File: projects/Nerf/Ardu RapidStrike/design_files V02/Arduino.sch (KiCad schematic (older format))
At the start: 51 parts, among them J1 BATT_IN, J10 MTR_2, J11 BATT_OUT, J12 CLIP, J13 NPTH, J14 NPTH, J16 NPTH, J2 BATT_IN, J3 PUSHER, J4 JAM, J5 I2C, J6 TRIGGER, J7 FTDI, J8 SENSORS, J9 MTR_1, Q1 IRLB8721, SW1 SW_Rotary8, SW2 SW_Push, U1 MCP1702, U2 L293D, U3 HALL SENSOR, U4 HALL SENSOR, U5 ATMEGA328P-PU, U6 HALL SENSOR, Y1 16Mhz

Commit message: Updates
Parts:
- removed J6: TRIGGER, Connectors_Molex:Molex_PicoBlade_53048-0610_06x1.25mm_Angled, symbol Conn_01x06
- removed SW2: SW_Push, footprints:SW_PUSH_6mm, symbol SW_Push
- added C9, C?: 0.1uF, footprints:C_Disc_D3.4mm_W2.1mm_P2.50mm, symbol C
- added J15: BATT, Connectors_Terminal_Blocks:TerminalBlock_bornier-2_P5.08mm, symbol Conn_01x02
- added J17: PSH_IN, footprints:Molex_PicoBlade_53048-0410_04x1.25mm_Angled, symbol Conn_01x04
- added J18: PSH_OUT, footprints:Molex_PicoBlade_53048-0410_04x1.25mm_Angled, symbol Conn_01x04
- added J?: TRIG, Pin_Headers:Pin_Header_Straight_2x01_Pitch2.00mm, symbol Conn_01x02
- added J?: REV, Pin_Headers:Pin_Header_Straight_2x01_Pitch2.00mm, symbol Conn_01x02
- added J?: PUSH, Pin_Headers:Pin_Header_Straight_2x01_Pitch2.00mm, symbol Conn_01x02
- added J?: BUTTON, Pin_Headers:Pin_Header_Straight_2x01_Pitch2.00mm, symbol Conn_01x02
- added J? (x2): TRIG_OUT, Connectors_Molex:Molex_PicoBlade_53048-0610_06x1.25mm_Angled, symbol Conn_01x06
- added R17, R?: 10K, footprints:R__P5.08mm, symbol R
- added R?: 1K, footprints:R__P5.08mm, symbol R
- added U7, U?: 74LS14, Housings_DIP:DIP-8_W7.62mm, symbol 74LS14
- J3: footprint footprints:TerminalBlock_Phoenix_PT-1,5-2-3.5-H_1x02_P3.50mm_Horizontal -> Connectors_Terminal_Blocks:TerminalBlock_bornier-2_P5.08mm
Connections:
- net labels added: #RTS, BUTTON, PUSHER, REV
- net labels removed: ACCEL, PUSH
- wire segments 209 -> 207
- no-connect marks 6 -> 5
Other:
- note removed: "DEBOUNCE"
- note removed: "PUSHER"
- moved on the sheet: C2, C3, C6, C7, C8, J12, J3, J5, J7, J8, R1, R10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

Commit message: Updates
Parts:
- removed J1: BATT_IN, footprints:TerminalBlock_Phoenix_PT-1,5-3-3.5-H_1x03_P3.50mm_Horizontal, symbol Conn_01x03
- removed J10: MTR_2, footprints:PhoenixContact_MCV-G_02x3.50mm_Vertical, symbol Conn_01x02
- removed J11: BATT_OUT, footprints:TerminalBlock_Phoenix_PT-1,5-3-3.5-H_1x03_P3.50mm_Horizontal, symbol Conn_01x03
- removed J13: NPTH, Wire_Pads:SolderWirePad_single_2-5mmDrill, symbol CONN_01X01
- removed J17: PSH_IN, footprints:Molex_PicoBlade_53048-0410_04x1.25mm_Angled, symbol Conn_01x04
- removed J18: PSH_OUT, footprints:Molex_PicoBlade_53048-0410_04x1.25mm_Angled, symbol Conn_01x04
- removed J8: SENSORS, Connectors_Molex:Molex_PicoBlade_53048-0510_05x1.25mm_Angled, symbol Conn_01x05
- added J1: BATT_OUT, Connectors_Terminal_Blocks:TerminalBlock_bornier-2_P5.08mm, symbol Conn_01x02
- added J10: PWM_IN, Pin_Headers:Pin_Header_Straight_1x01_Pitch2.00mm, symbol CONN_01X01
- added J11: PWM_OUT, Pin_Headers:Pin_Header_Straight_1x01_Pitch2.00mm, symbol CONN_01X01
- added J17: PSH_IN, Connectors_Molex:Molex_PicoBlade_53048-0510_05x1.25mm_Angled, symbol Conn_01x05
- added J18: PSH_OUT, Connectors_Molex:Molex_PicoBlade_53048-0510_05x1.25mm_Angled, symbol Conn_01x05
- added J8: DART, Connectors_Molex:Molex_PicoBlade_53048-0310_03x1.25mm_Angled, symbol CONN_01X03
- added LS1: Speaker, footprints:SPEAKER, symbol Speaker
- J2: footprint footprints:TerminalBlock_Phoenix_PT-1,5-2-5.0-H_1x02_P5.00mm_Horizontal -> footprints:XT30PW_M
- J23: renamed from J?; value TRIG_OUT -> TRIG_IN
- J9: value MTR_1 -> MTR; footprint footprints:PhoenixContact_MCV-G_02x3.50mm_Vertical -> footprints:XT30PW_F
- U7: footprint Housings_DIP:DIP-8_W7.62mm -> footprints:DIP-14_W7.62mm
- gave numbers to parts that had none: 9
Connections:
- net labels added: DB_GND, DB_VCC
- wire segments 207 -> 208
- no-connect marks 5 -> 4
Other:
- note added: "A0 BUTTON\nA1 CLIP\nA2 FIRE SEL\nA3 Voltage\n\n"
- note added: "D2 Pusher SW\nD3 DART IR\nD4 SPKR\nD5 Pusher A\nD6 Pusher B\nD7 Rev SW\nD8 Trig SW\nD9 Flywheel\nD10 Clip U3\nD11 Clip U4\nD12 Clip U6\nD13 LED"
- note removed: "+\n-\nS"
- note removed: "A0 -\nA1 CLIP\nA2 FIRE SEL\nA3 Voltage\n\n"
- note removed: "D2 INT pin 1\nD3 INT pin 2\nD4 Pusher SW\nD5 Pusher A\nD6 Pusher B\nD7 Rev SW\nD8 Trig SW\nD9 Flywheel\nD10 Clip U3\nD11 Clip U4\nD12 Clip U6\nD13 LED"
- note removed: "SIG\n+\n -\n\n"
- moved on the sheet: C1, C10, C2, C3, C4, C5, C6, C7, C8, C9, D1, D2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

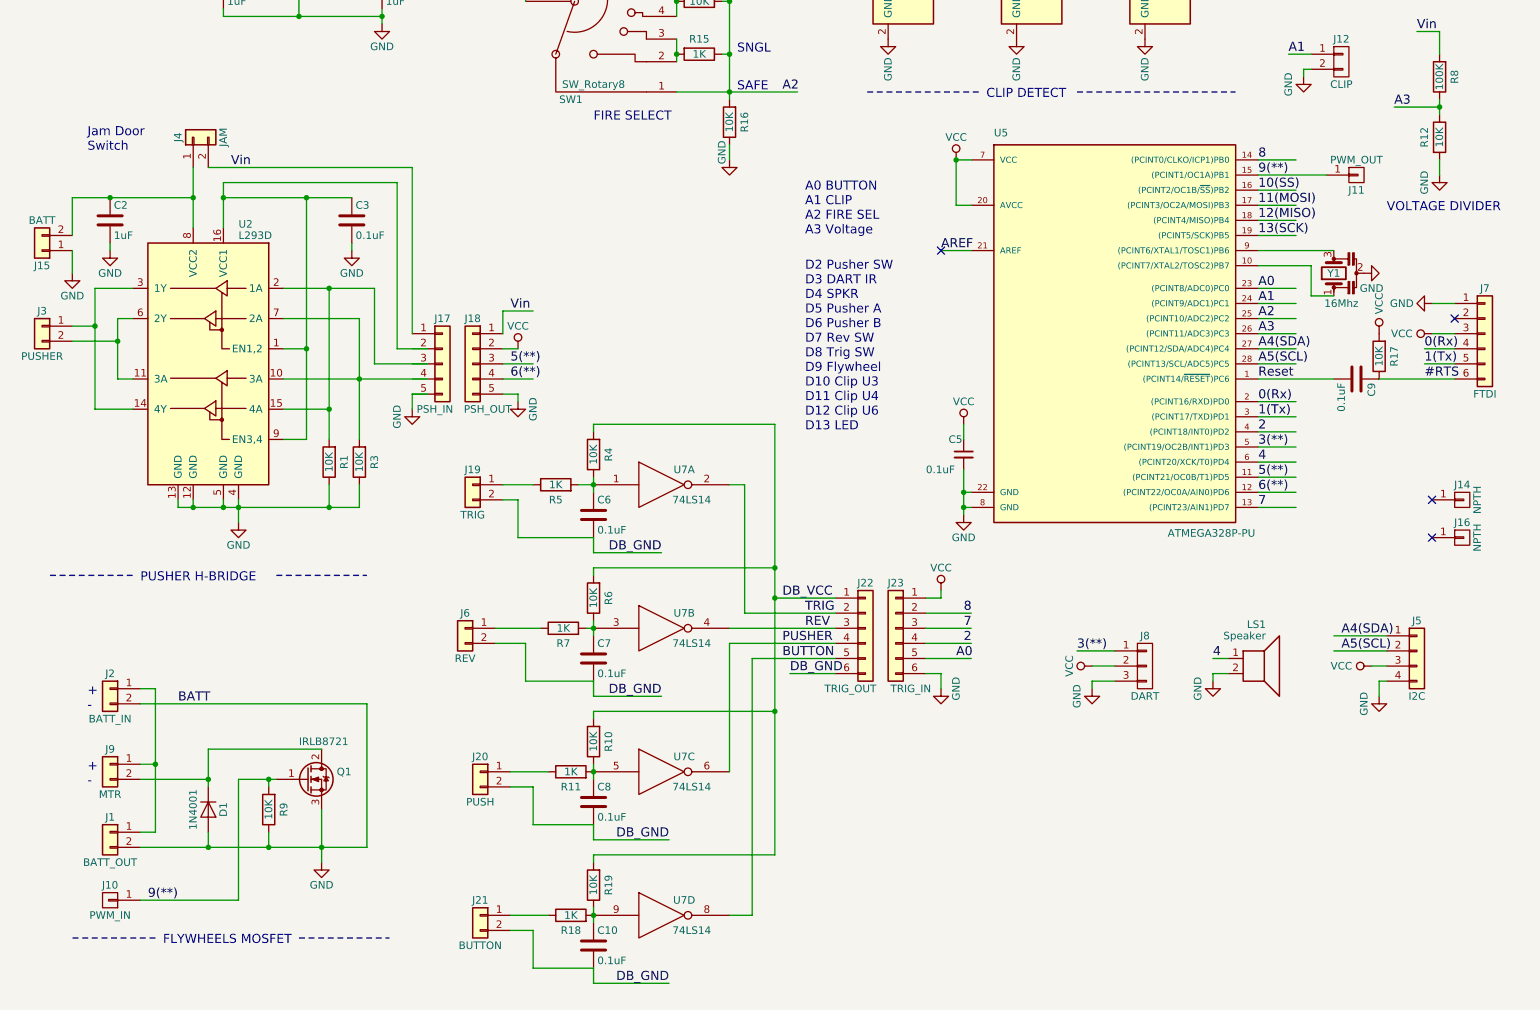
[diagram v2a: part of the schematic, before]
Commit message: Iupdates
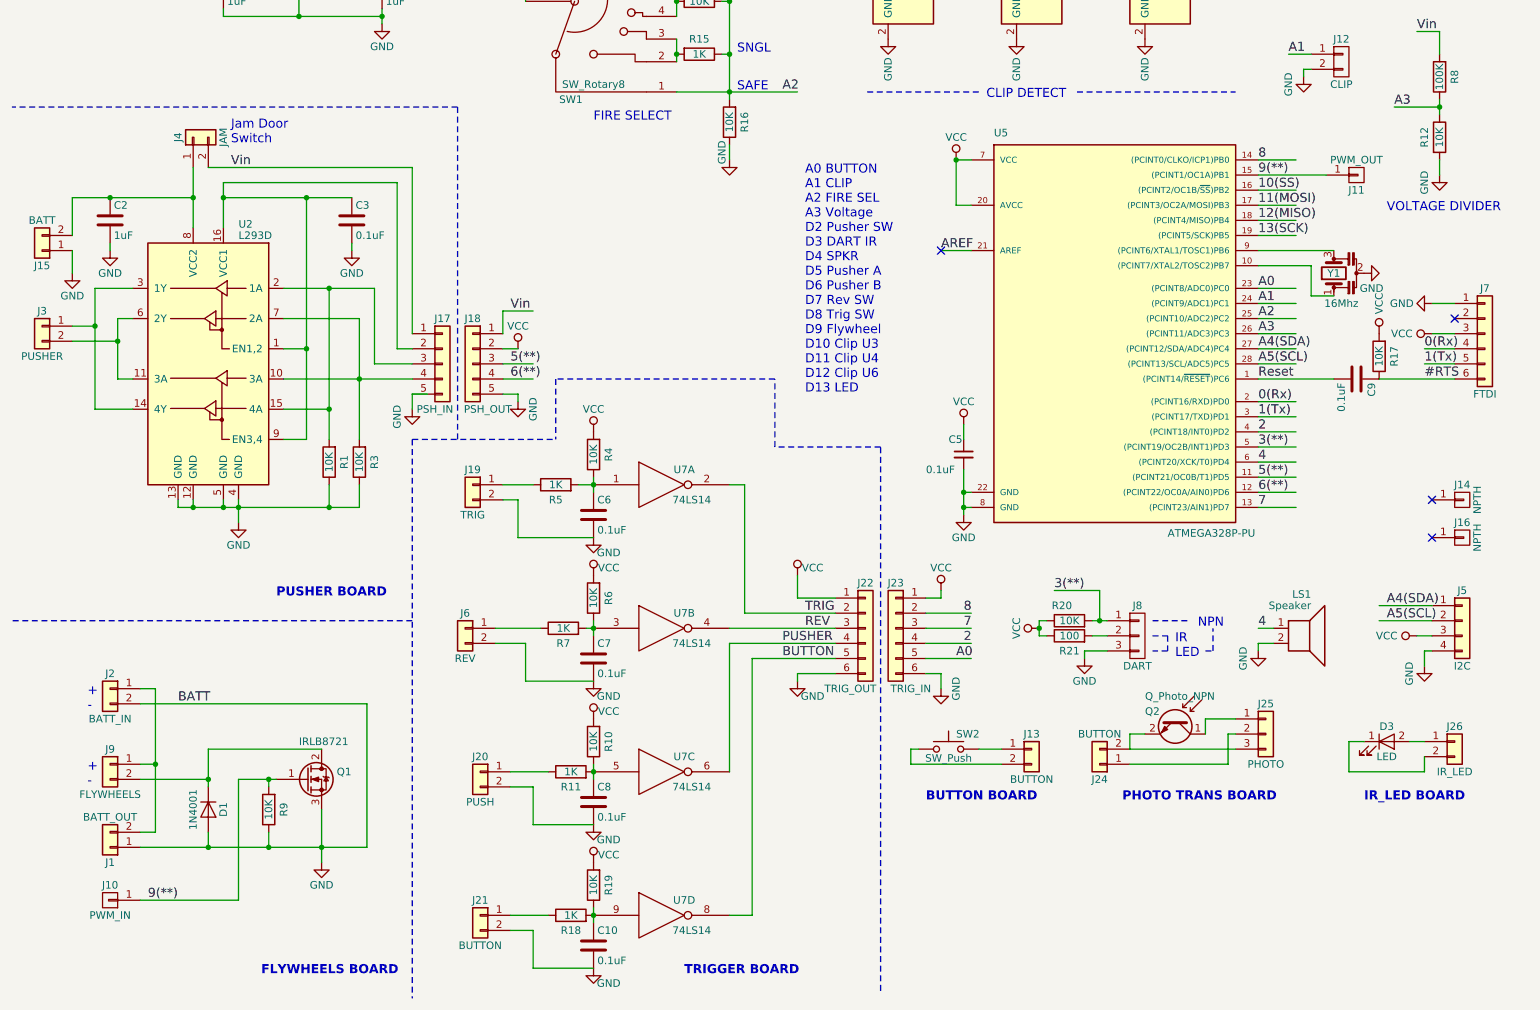
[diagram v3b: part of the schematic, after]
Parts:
- added D3: LED, footprints:LED_D3.0mm, symbol LED
- added J13, J24: BUTTON, Pin_Headers:Pin_Header_Straight_1x02_Pitch2.00mm, symbol Conn_01x02
- added J25: PHOTO, Pin_Headers:Pin_Header_Straight_1x03_Pitch2.00mm, symbol Conn_01x03
- added J26: IR_LED, Pin_Headers:Pin_Header_Straight_1x02_Pitch2.00mm, symbol Conn_01x02
- added Q2: Q_Photo_NPN, symbol Q_Photo_NPN
- added R20: 10K, footprints:R__P5.08mm, symbol R
- added R21: 100, footprints:R__P5.08mm, symbol R
- added SW2: SW_Push, footprints:SW_PUSH_6mm, symbol SW_Push
- J9: value MTR -> FLYWHEELS
- U7: footprint Housings_DIP:DIP-8_W7.62mm -> footprints:DIP-14_W7.62mm
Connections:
- net labels removed: DB_GND, DB_VCC
- wire segments 208 -> 215
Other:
- note added: "A0 BUTTON\nA1 CLIP\nA2 FIRE SEL\nA3 Voltage\nD2 Pusher SW\nD3 DART IR\nD4 SPKR\nD5 Pusher A\nD6 Pusher B\nD7 Rev SW\nD8 Trig SW\nD9 Flywheel\nD10 Clip U3\nD11 Clip U4\nD12 Clip U6\nD13 LED"
- note added: "BUTTON BOARD"
- note added: "FLYWHEELS BOARD"
- note added: "IR\nLED"
- note added: "IR_LED BOARD"
- note added: "NPN"
- note added: "PHOTO TRANS BOARD"
- note added: "PUSHER BOARD"
- note added: "TRIGGER BOARD"
- note removed: "A0 BUTTON\nA1 CLIP\nA2 FIRE SEL\nA3 Voltage\n\n"
- note removed: "D2 Pusher SW\nD3 DART IR\nD4 SPKR\nD5 Pusher A\nD6 Pusher B\nD7 Rev SW\nD8 Trig SW\nD9 Flywheel\nD10 Clip U3\nD11 Clip U4\nD12 Clip U6\nD13 LED"
- note removed: "FLYWHEELS MOSFET"
- note removed: "PUSHER H-BRIDGE"
- moved on the sheet: J5, J8, LS1
